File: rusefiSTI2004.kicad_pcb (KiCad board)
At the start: 2 copper layers, 138.4 x 76.4 mm, 2 parts, among them M100 Module:mega_mcu100-f7/0.2, M1000 Module:mega_mcu144/0.7

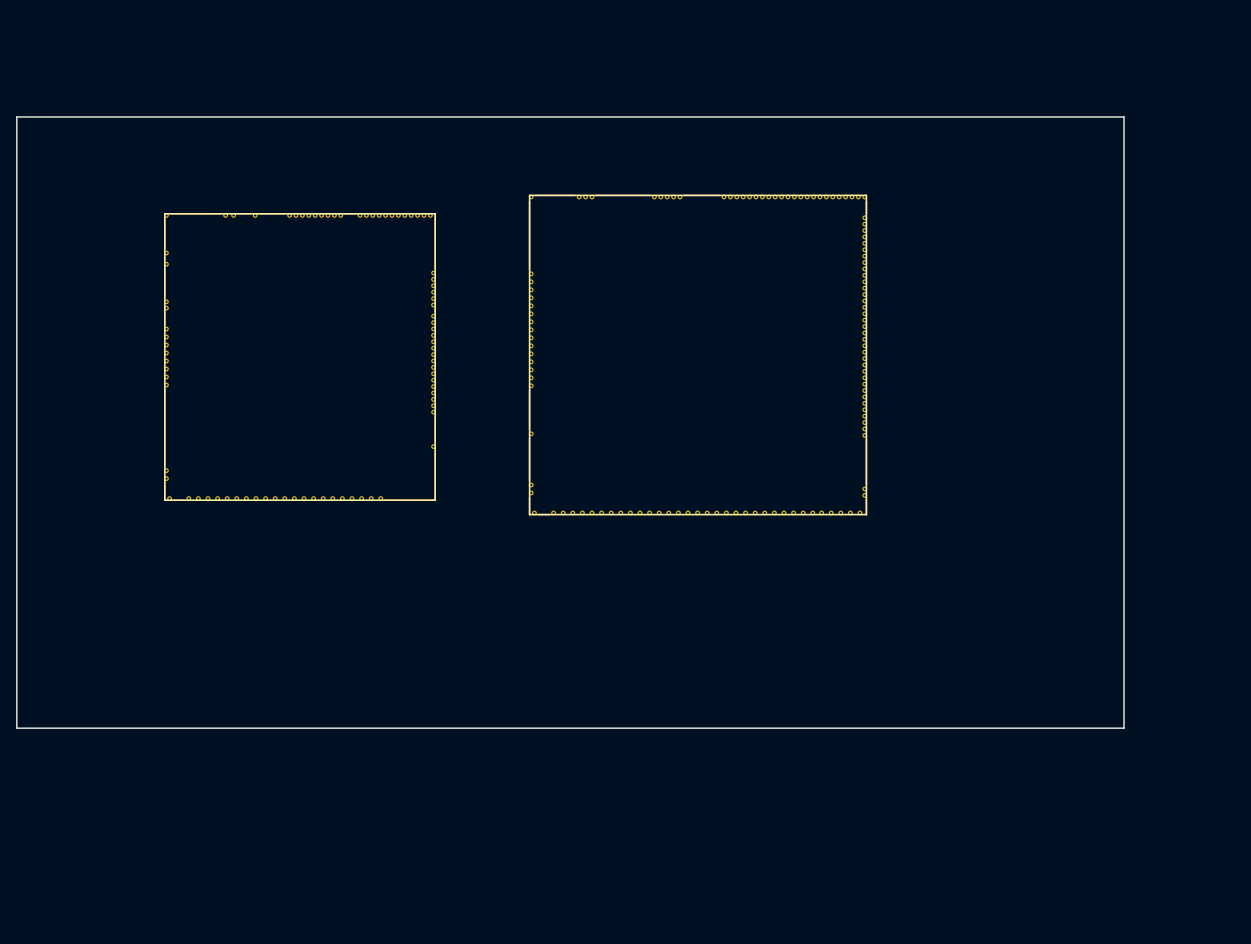
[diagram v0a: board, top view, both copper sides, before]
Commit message: started laying it out
quick layout
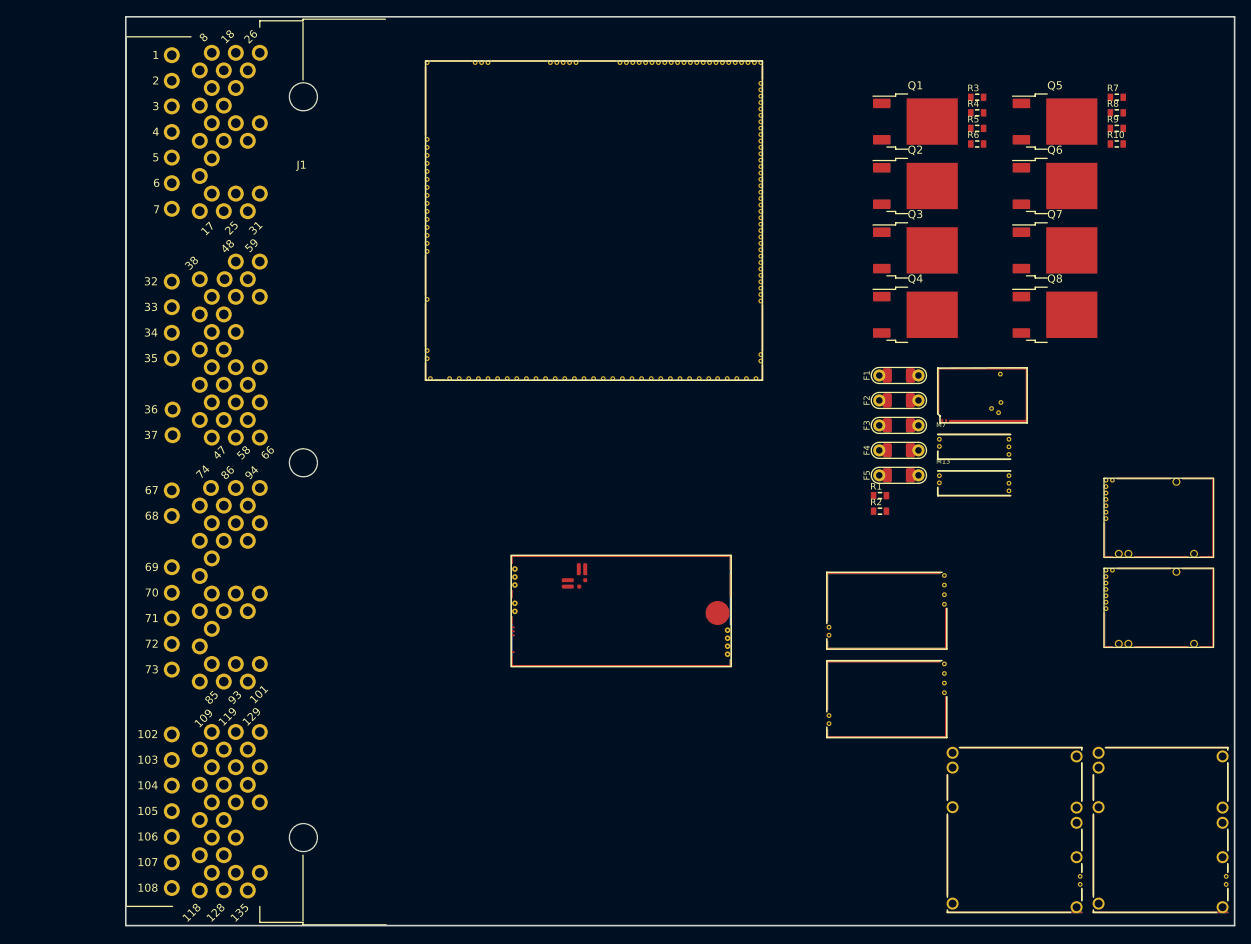
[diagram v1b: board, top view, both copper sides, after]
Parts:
- removed M100: Module:mega_mcu100-f7/0.2, Module-mega-mcu100-f7/0.2:mega-mcu100-f7
- removed M1000: Module:mega_mcu144/0.7, AAmega-mcu144:mega-mcu144
- added F1: nSMD005, hellen-one-common:PAD-1206-PAD, F.Cu at (181.9, 80.7)
- added F2: nSMD005, hellen-one-common:PAD-1206-PAD, F.Cu at (181.9, 83.8)
- added F3: nSMD005, hellen-one-common:PAD-1206-PAD, F.Cu at (181.9, 86.9)
- added F4: nSMD005, hellen-one-common:PAD-1206-PAD, F.Cu at (181.9, 90.1)
- added F5: nSMD005, hellen-one-common:PAD-1206-PAD, F.Cu at (181.9, 93.2)
- added J1: 1-1376430-0, STI:1-1376430-0, F.Cu at (91.0, 40.4)
- added M1: Module-mega-mcu144-0.7, hellen-one-mega-mcu144-0.7:mega-mcu144, F.Cu at (122.6, 81.4)
- added M13: Module-knock-0.2, hellen-one-knock-0.2:knock, F.Cu at (186.6, 95.8)
- added M14: Module-power_12and5V-0.3, hellen-one-power_12and5V-0.3:power_12and5V, F.Cu at (206.1, 147.9)
- added M2: Module-motor-driver-0.1, hellen-one-motor-driver-0.1:motor-driver, F.Cu at (207.4, 103.5)
- added M3: Module-wbo-0.5, hellen-one-wbo-0.5:wbo, F.Cu at (133.3, 117.2)
- added M4: Module-can-0.1, hellen-one-can-0.1:can, F.Cu at (186.6, 86.7)
- added M5: Module-vr-discrete-0.5, hellen-one-vr-discrete-0.5:vr-discrete, F.Cu at (172.8, 115.0)
- added M6: Module-vr-discrete-0.5, hellen-one-vr-discrete-0.5:vr-discrete, F.Cu at (172.8, 126.1)
- added M7: Module-knock-0.2, hellen-one-knock-0.2:knock, F.Cu at (186.6, 91.3)
- added M8: Module-power_12and5V-0.3, hellen-one-power_12and5V-0.3:power_12and5V, F.Cu at (187.8, 147.9)
- added M9: Module-motor-driver-0.1, hellen-one-motor-driver-0.1:motor-driver, F.Cu at (207.4, 114.7)
- added Q1: VND14NV04-E, hellen-one-common:DPAK, F.Cu at (182.8, 49.0)
- added Q2: VND14NV04-E, hellen-one-common:DPAK, F.Cu at (182.8, 57.0)
- added Q3: VND14NV04-E, hellen-one-common:DPAK, F.Cu at (182.8, 65.1)
- added Q4: VND14NV04-E, hellen-one-common:DPAK, F.Cu at (182.8, 73.1)
- added Q5: VND14NV04-E, hellen-one-common:DPAK, F.Cu at (200.3, 49.0)
- added Q6: VND14NV04-E, hellen-one-common:DPAK, F.Cu at (200.3, 57.0)
- added Q7: VND14NV04-E, hellen-one-common:DPAK, F.Cu at (200.3, 65.1)
- added Q8: VND14NV04-E, hellen-one-common:DPAK, F.Cu at (200.3, 73.1)
- added R1: 33k, hellen-one-common:R0603, F.Cu at (179.5, 95.7)
- added R10: 4.7k, hellen-one-common:R0603, F.Cu at (209.1, 51.8)
- added R2: 6.8k, hellen-one-common:R0603, F.Cu at (179.5, 97.7)
- added R3: 4.7k, hellen-one-common:R0603, F.Cu at (191.7, 45.9)
- added R4: 4.7k, hellen-one-common:R0603, F.Cu at (191.7, 47.9)
- added R5: 4.7k, hellen-one-common:R0603, F.Cu at (191.7, 49.8)
- added R6: 4.7k, hellen-one-common:R0603, F.Cu at (191.7, 51.8)
- added R7: 4.7k, hellen-one-common:R0603, F.Cu at (209.1, 45.9)
- added R8: 4.7k, hellen-one-common:R0603, F.Cu at (209.1, 47.9)
- added R9: 4.7k, hellen-one-common:R0603, F.Cu at (209.1, 49.8)
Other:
- board size 138.4 x 76.4 mm -> 138.6 x 113.6 mm
